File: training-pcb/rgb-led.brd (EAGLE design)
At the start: 30 x 30 mm, 24 parts, among them J1 MICRO-USB, J2 AVR_SPI_PROG2PTH2, K1 SKQGADE010, U1 ATTINY441/841SSU/SSUR, U2 PCA9533

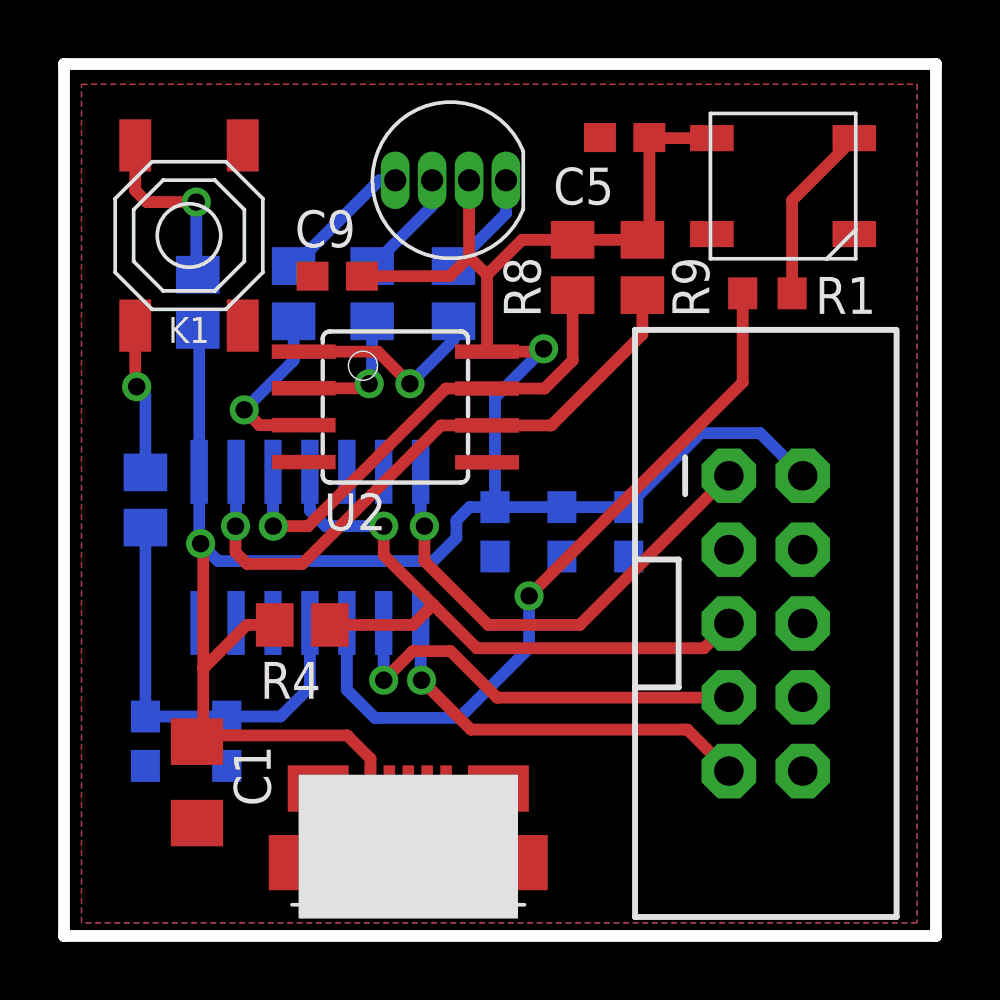
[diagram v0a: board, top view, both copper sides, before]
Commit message: Minor PCB changes, change resistor sizes
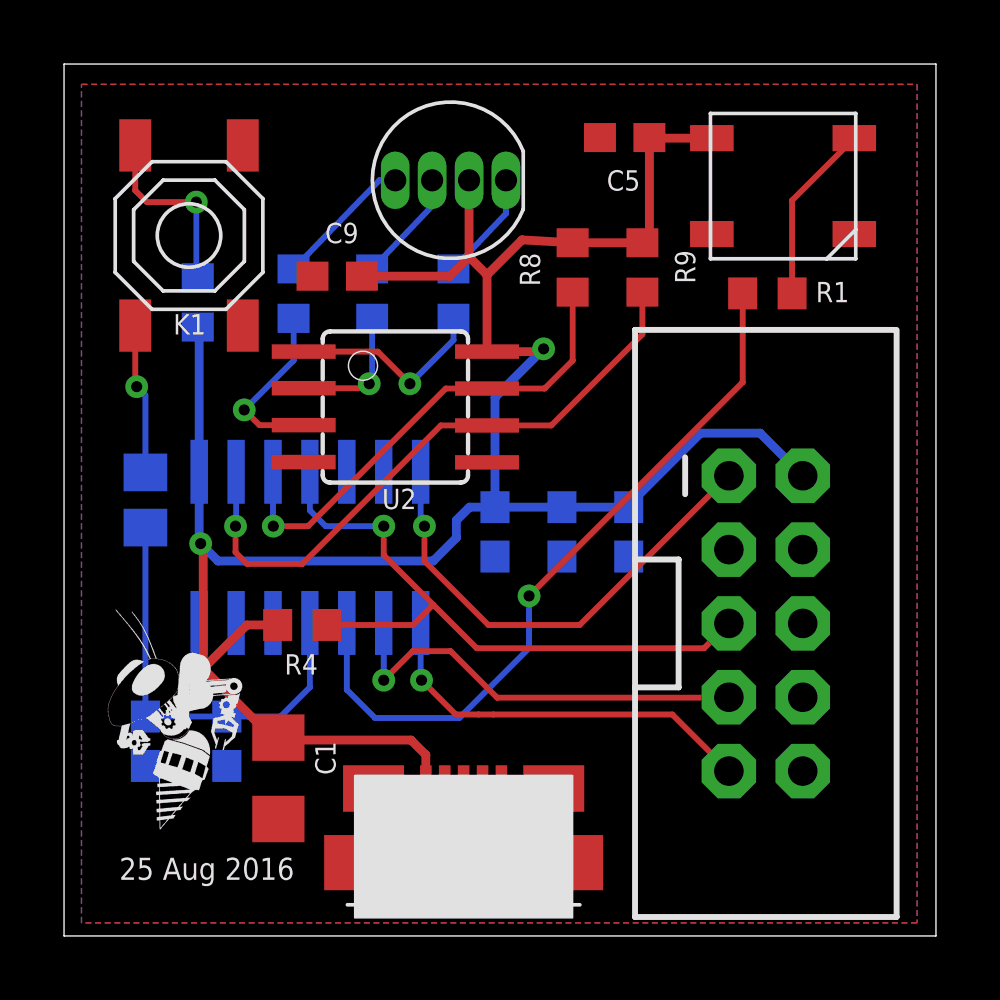
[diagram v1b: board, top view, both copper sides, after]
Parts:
- added U$2: (no value), RoboJackets-Aesthetics:ROBOBUZZ_0.4X
- C1: value 100u -> 47u
- R2, R4, R5, R6, R7, R8, R9: device resistor:R0805 -> resistor:R0603
- moved C1 2.80 mm to (7.37, 5.42)
- moved J1 1.91 mm to (13.7, 2.52)
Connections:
- net GND: now also J1.5@1, J1.5@2, J1.5@3, J1.5@4, J1.5@6, J1.5@7
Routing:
- net +5V: track 78.1 -> 78.9 mm
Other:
- board text added: "25 Aug 2016"
